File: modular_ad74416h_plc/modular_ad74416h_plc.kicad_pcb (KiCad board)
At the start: 2 copper layers, 45.7 x 2.5 mm, 8 parts

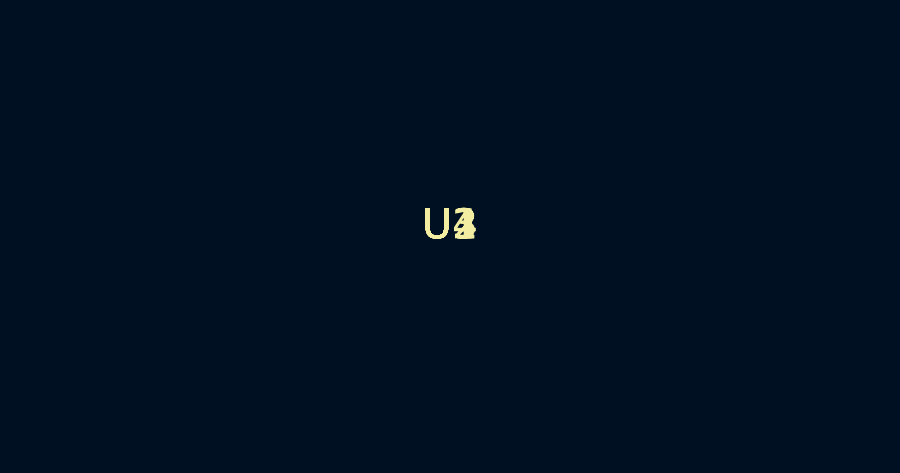
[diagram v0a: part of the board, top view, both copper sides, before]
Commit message: backup
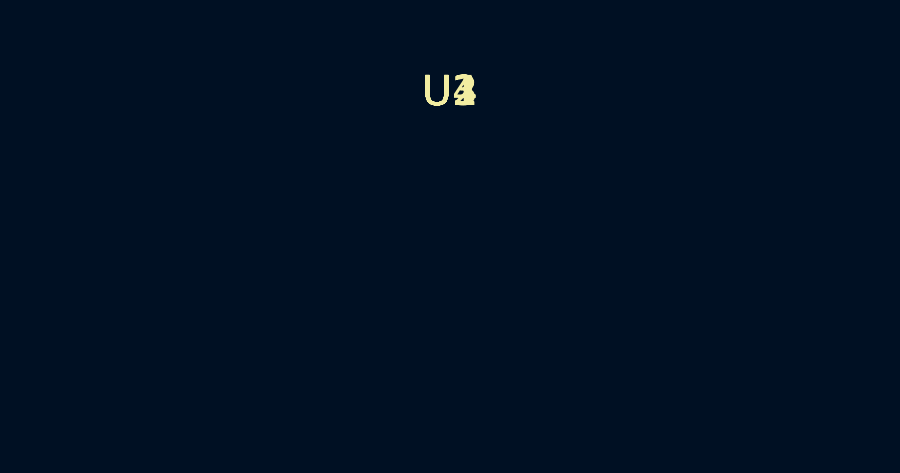
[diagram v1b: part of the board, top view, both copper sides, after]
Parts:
- moved U1 4.44 mm to (193.8, 120.5)
- moved U2 4.44 mm to (193.8, 120.5)
- moved U3 4.44 mm to (193.8, 120.5)
- moved U4 4.44 mm to (193.8, 120.5)
- moved MOD2 0.25 mm to (193.8, 172.4)
- moved MOD5 0.25 mm to (210.3, 166.8)
- moved MOD1 0.25 mm to (193.8, 158.6)

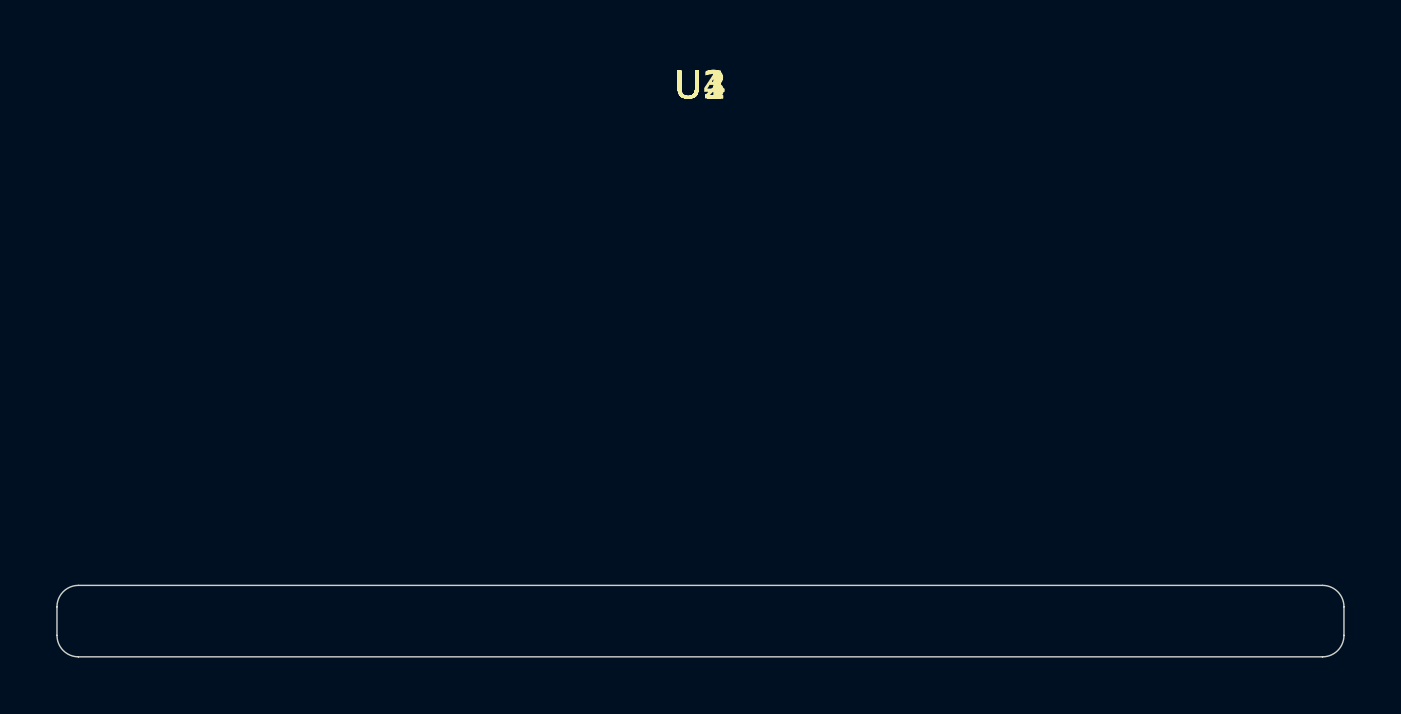
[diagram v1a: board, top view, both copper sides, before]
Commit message: backup
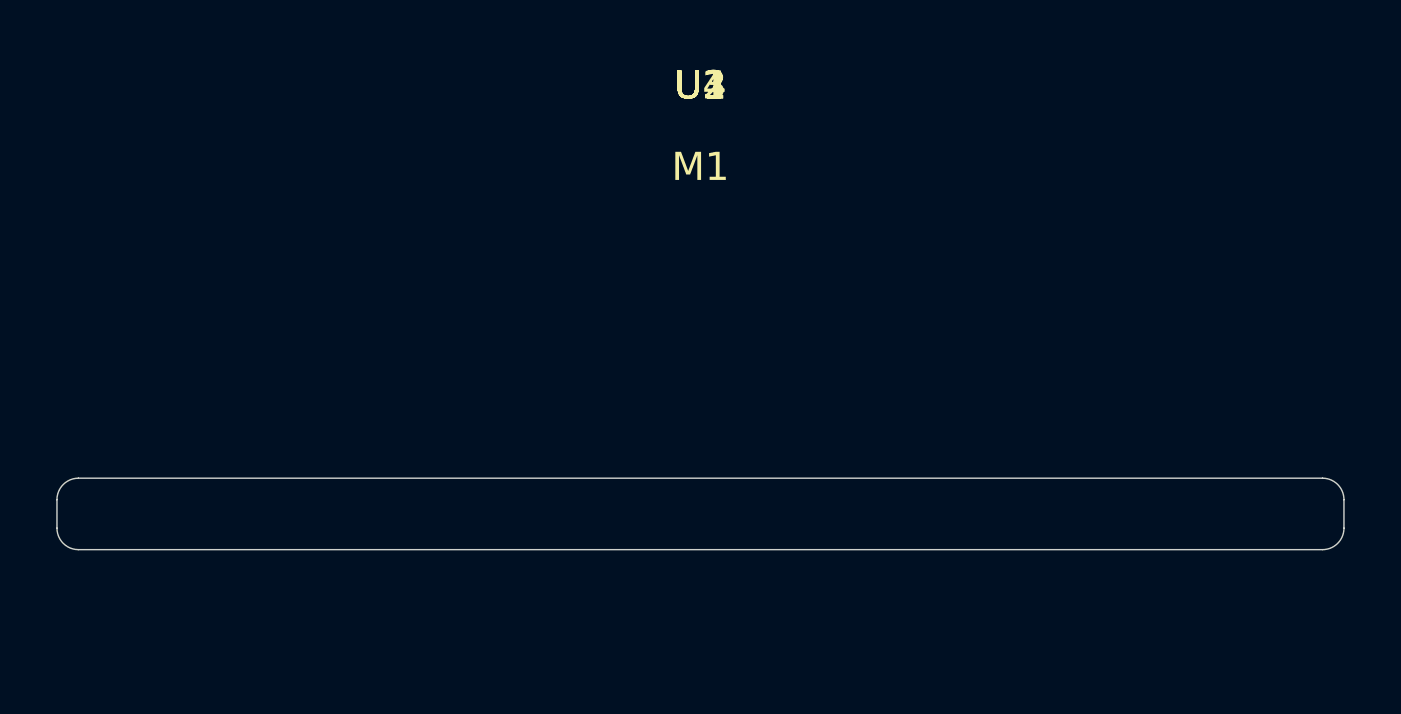
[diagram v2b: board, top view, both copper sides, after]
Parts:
- added M1: ~, mechanical_parts:2203350, F.Cu at (193.8, 123.4)

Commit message: Update kicad-config.yml and modular_ad74416h_plc.kicad_pcb
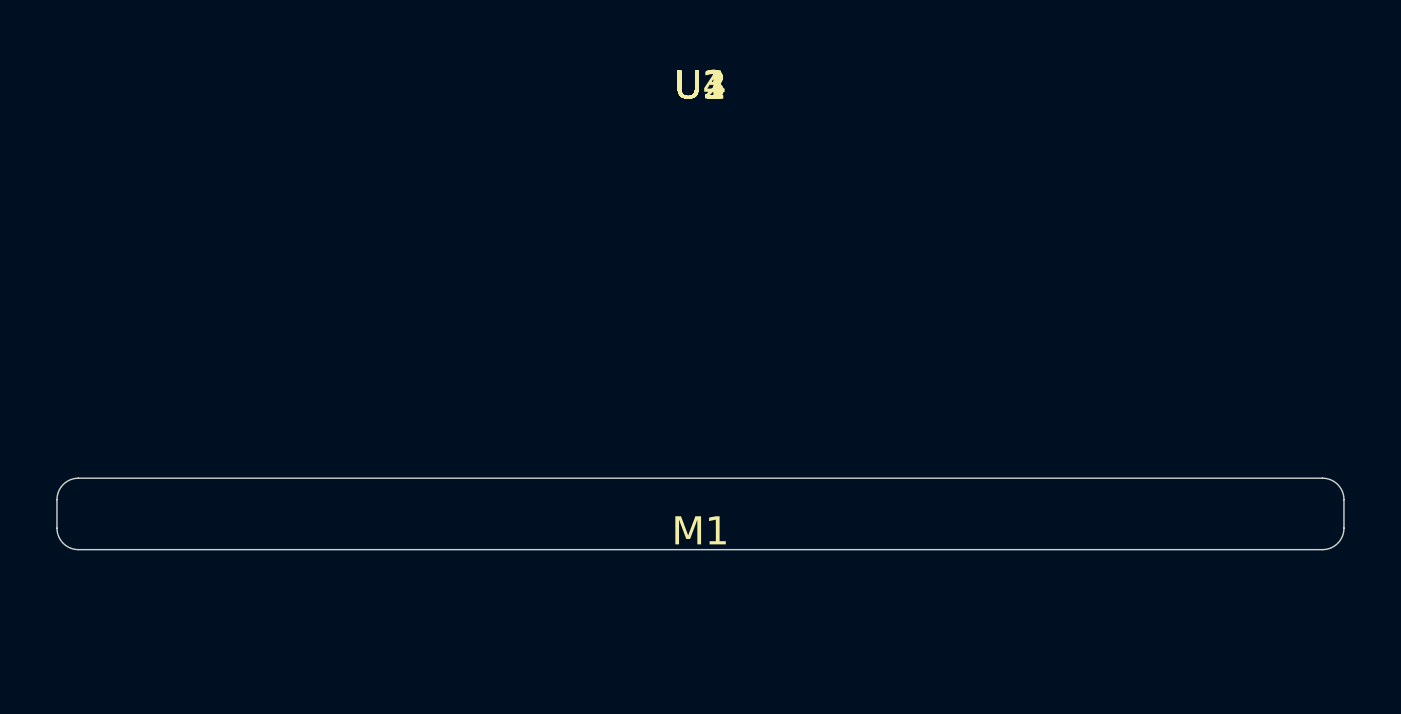
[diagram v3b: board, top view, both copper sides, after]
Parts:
- moved M1 13.0 mm to (193.8, 136.4)
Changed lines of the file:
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@@
 	(footprint "mechanical_parts:2203350"
 		(layer "F.Cu")
-		(at 193.8274 123.444)
+		(at 193.8274 136.398)
 		(descr "UCS HH 125-87 9005 - Housing half shell")
 		(property "Reference" "M1"
@@
 		(model "${KICAD9_3D_MODELS_VAULT}/3D_models/mechanical/2203350.step"
 			(offset
-				(xyz 0 0 0)
+				(xyz 0 0 -13.335)
 			)
 			(scale
@@
 			)
 			(rotate
-				(xyz 0 0 0)
-			)
-		)
+				(xyz -0 -0 -0)
+			)
+		)

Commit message: backup
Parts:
- added M2: ~, mechanical_parts:2203404_v2, F.Cu at (158.6, 82.2)
- added M3: ~, mechanical_parts:2203404_v2, F.Cu at (229.0, 82.2)
- added M4: ~, mechanical_parts:2203404_v2, F.Cu at (158.6, 190.6)
- added M5: ~, mechanical_parts:2203404_v2, F.Cu at (229.0, 190.6)

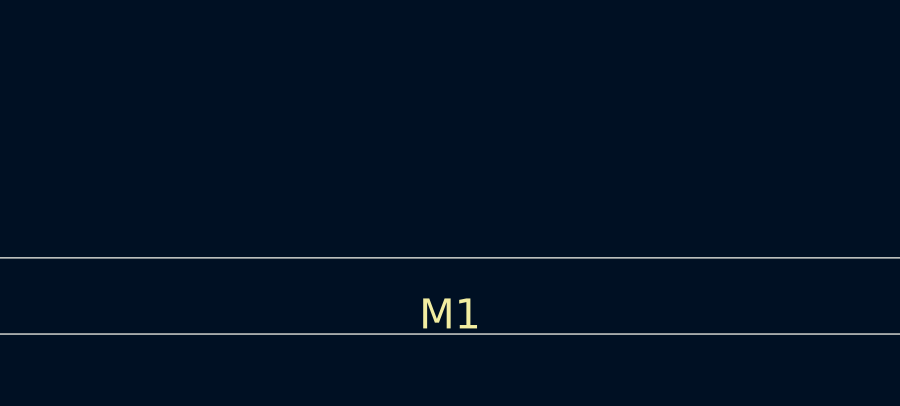
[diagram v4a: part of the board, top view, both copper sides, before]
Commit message: backup
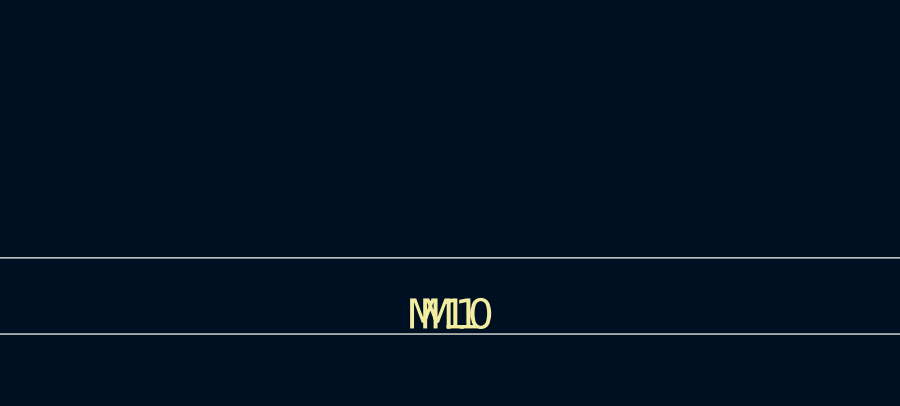
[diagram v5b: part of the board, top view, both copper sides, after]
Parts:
- added M10: ~, mechanical_parts:2203350, F.Cu at (193.8, 136.4)
- added M6: ~, mechanical_parts:2203400, F.Cu at (229.0, 82.2)
- added M7: ~, mechanical_parts:2203400, F.Cu at (158.6, 82.2)
- added M8: ~, mechanical_parts:2203400, F.Cu at (158.6, 190.6)
- added M9: ~, mechanical_parts:2203400, F.Cu at (229.0, 190.6)
